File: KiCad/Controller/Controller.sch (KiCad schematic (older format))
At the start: 90 parts, among them IC2 ATXMEGA128A3-A, P1 PowerControl, P10 TapeLoopControl, P11 InputSelectorSwitch, P12 MainPowerTrigger, P2 PowerAmpMute, P3 SPowerAmpMute, P4 PDI, P5 CurrentSense, P6 InputSelect, P7 VolumeCtrl, P8 Power, P9 MetterCurrent, Q1 BC817-40, Q2 BC817-40, SW1 SW_DIP_x01, U1 L78L33, U2 INA169, U3 ILD217, U4 ISO7241A, U5 ISO1541, U6 LM358, U7 LTV-357Ts

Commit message: Refresh commit
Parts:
- C1, C11, C17, C19, C29, C4, C6, C8: symbol CP -> Device:CP
- C10, C12, C13, C14, C15, C16, C18, C2, C20, C21, C22, C23, C24, C25, C26, C27, C28, C3, C5, C7, C9: symbol C -> Device:C
- D1, D2: symbol LED-RESCUE-Controller -> Controller-rescue:LED-RESCUE-Controller
- IC2: symbol ATXMEGA128A3-A -> Controller-rescue:ATXMEGA128A3-A
- L1, L2: symbol L_Small -> Device:L_Small
- P1, P10, P5: symbol CONN_01X04 -> Controller-rescue:CONN_01X04
- P11, P12, P2, P3, P8, P9: symbol CONN_01X02 -> Controller-rescue:CONN_01X02
- P4: symbol CONN_02X03 -> Controller-rescue:CONN_02X03
- P6: symbol CONN_01X10 -> Controller-rescue:CONN_01X10
- P7: symbol CONN_02X04 -> Controller-rescue:CONN_02X04
- Q1, Q2: symbol BC817-40 -> Controller-rescue:BC817-40
- R1, R10, R11, R12, R13, R14, R15, R16, R17, R18, R19, R2, R20, R21, R22, R23, R24, R25, R26, R27, R28, R29, R3, R30, R31, R32, R4, R5, R6, R7, R8, R9: symbol R -> Device:R
- ROT1, ROT2: symbol ROTARY-ENCODER -> sparkfun:ROTARY-ENCODER
- SW1: symbol SW_DIP_x01-RESCUE-Controller -> Controller-rescue:SW_DIP_x01-RESCUE-Controller
- U1: symbol MC78L05ACH -> Controller-rescue:MC78L05ACH
- U2: symbol INA169 -> myLib:INA169
- U3: symbol LTV-827 -> Controller-rescue:LTV-827
- U4: symbol ISO7241 -> myLib:ISO7241
- U5: symbol ISO1541 -> myLib:ISO1541
- U6: symbol LM358 -> Controller-rescue:LM358
- U7: symbol LTV-357Ts -> myLib:LTV-357Ts

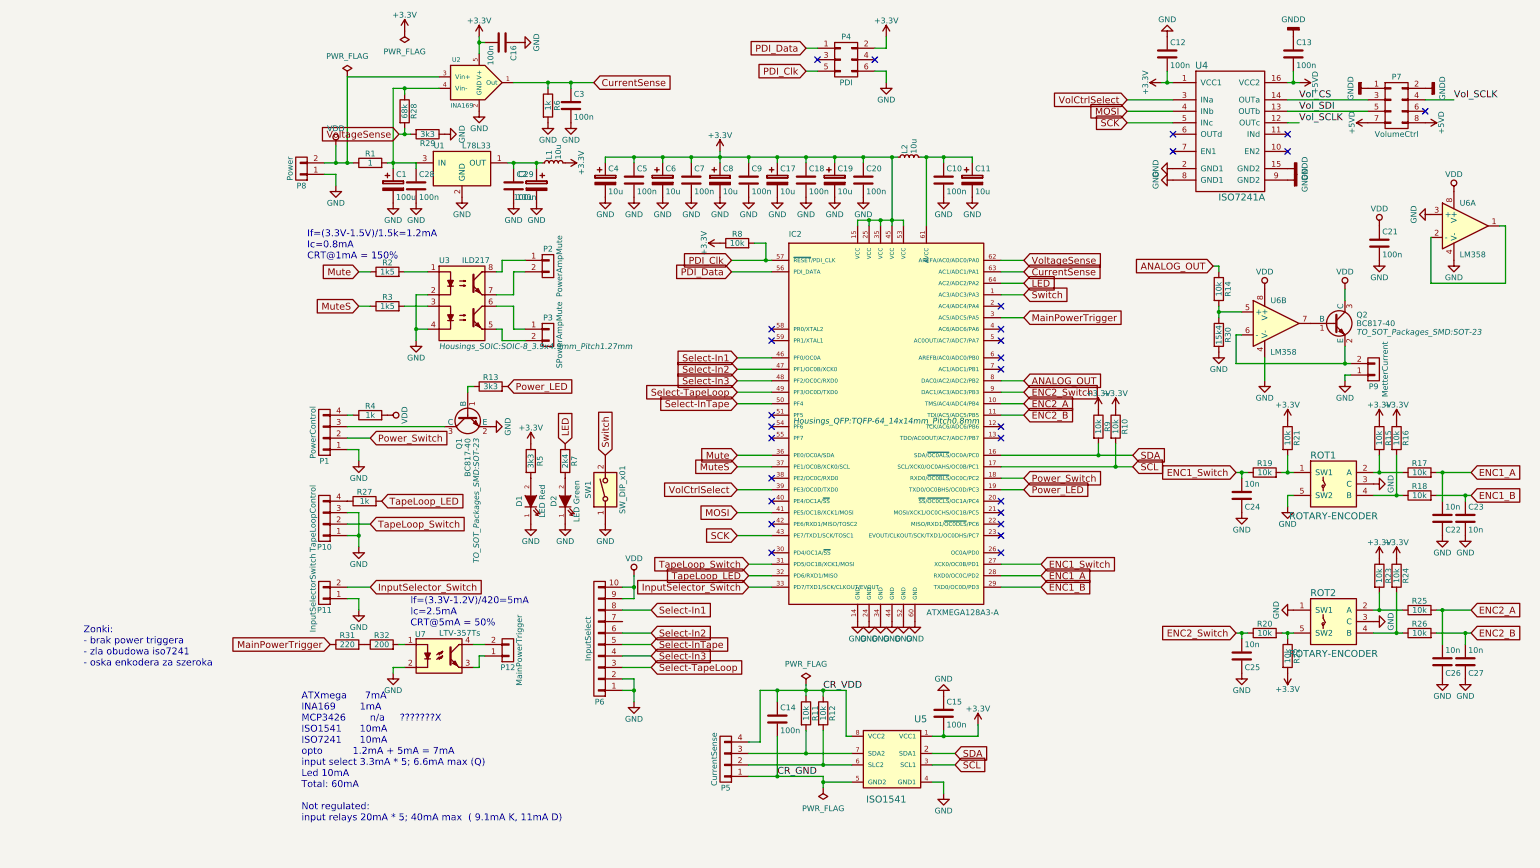
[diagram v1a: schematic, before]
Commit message: Commit
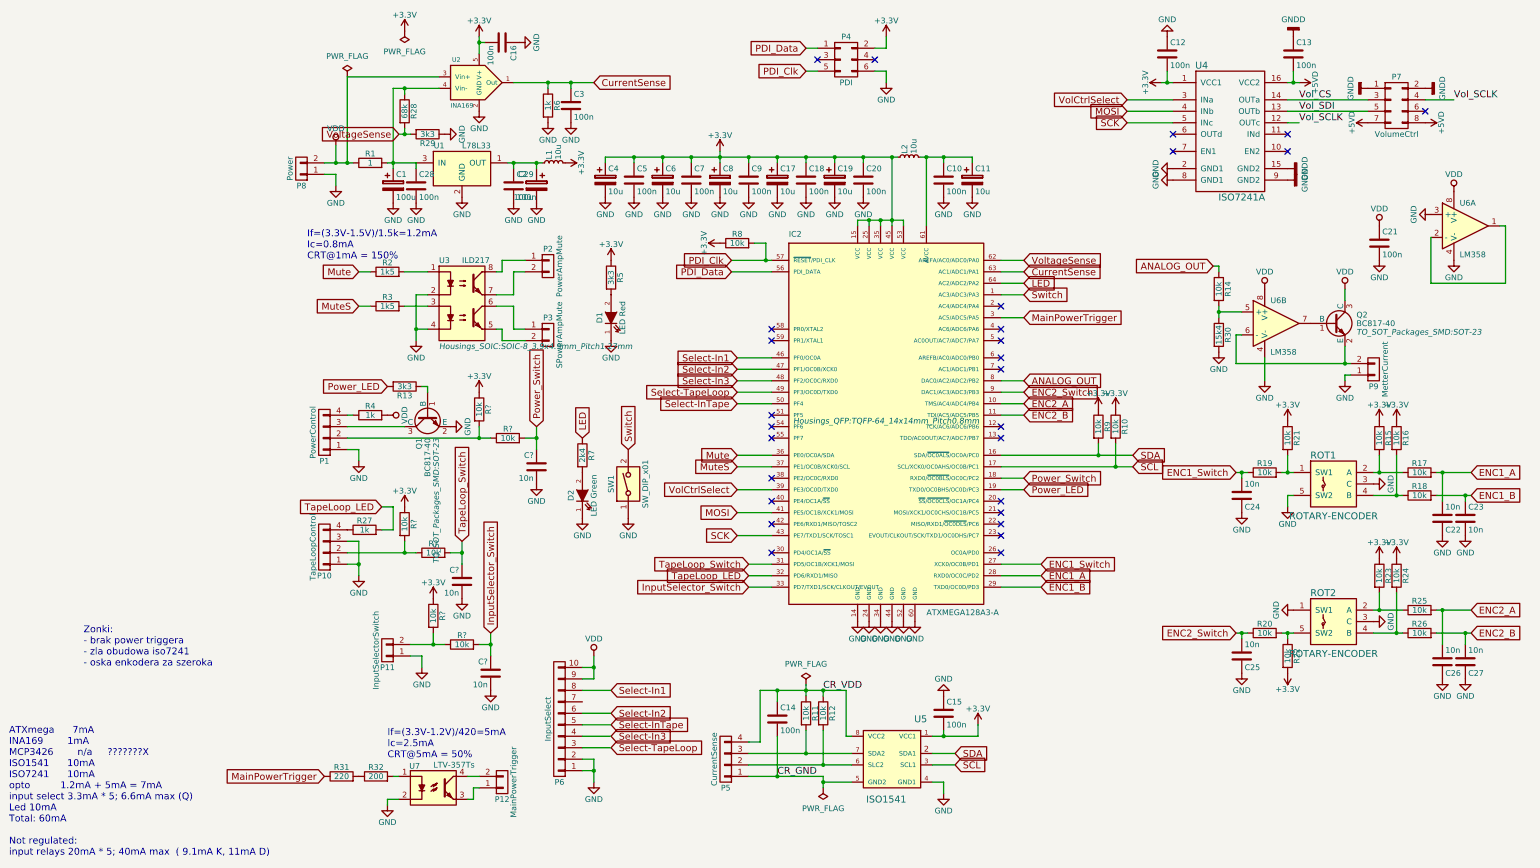
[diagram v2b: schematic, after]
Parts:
- added C? (x3): 10n, Capacitors_SMD:C_0805, symbol Device:C
- added R? (x6): 10k, Resistors_SMD:R_0805, symbol Device:R
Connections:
- net +3V3: now also R?.1, R?.1, R?.1
- net GND: now also C?.2, C?.2, C?.2
- net InputSelector_Switch: now also C?.1, R?.2; no longer P11.2 (P2)
- net Power_Switch: now also C?.1, R?.2; no longer P1.2 (P2)
- net TapeLoop_Switch: now also C?.1, R?.2; no longer P10.2 (P2)
- new net: P1.2 (P2), R?.1, R?.2
- new net: P10.2 (P2), R?.1, R?.2
- new net: P11.2 (P2), R?.1, R?.2
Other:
- moved on the sheet: D1, D2, P10, P11, P12, P6, Q1, R13, R27, R31, R32, R5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
